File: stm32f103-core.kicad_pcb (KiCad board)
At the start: 2 copper layers, 30 x 35 mm, 31 parts, among them J1 Conn_01x14, J3 Conn_01x12, J4 Conn_01x12, SW1 SW_Push, U1 STM32F103C8T6, U2 AMS1117-3.3, Y1 O8M, Y2 O32.768K

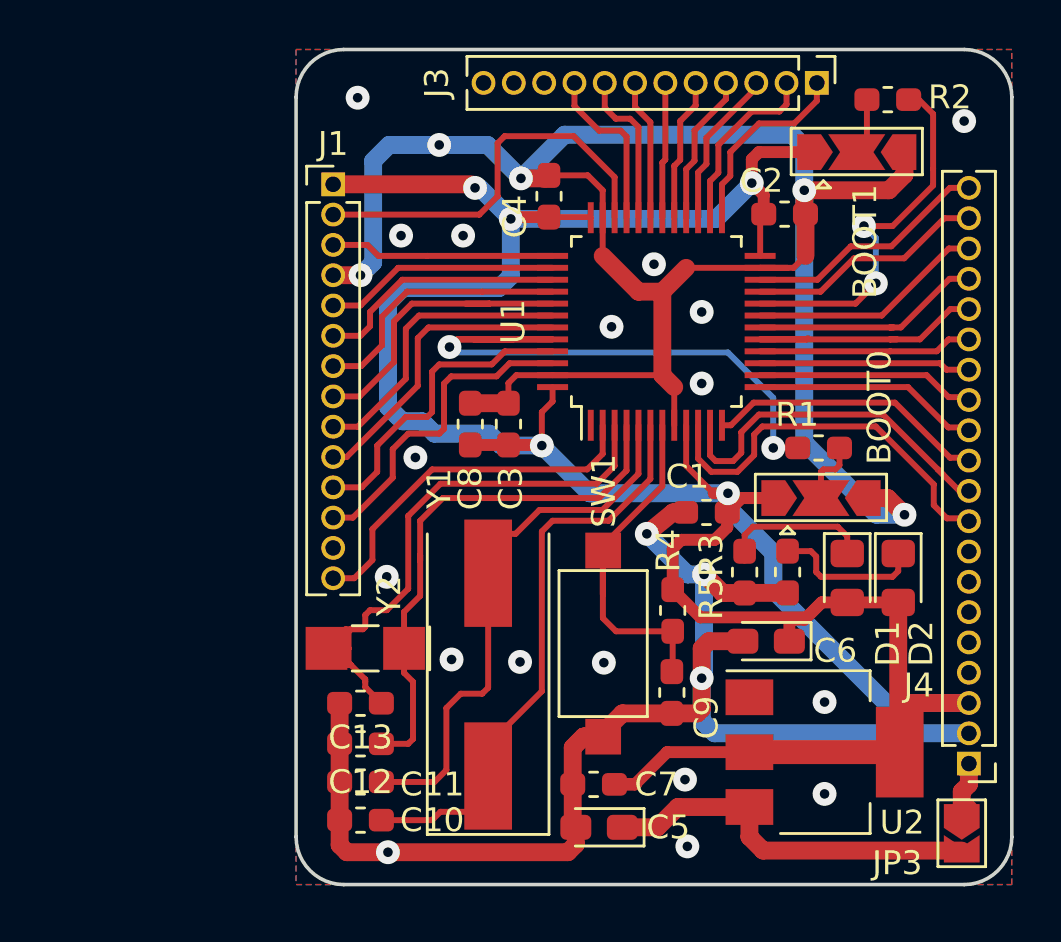
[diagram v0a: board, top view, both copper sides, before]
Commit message: update,
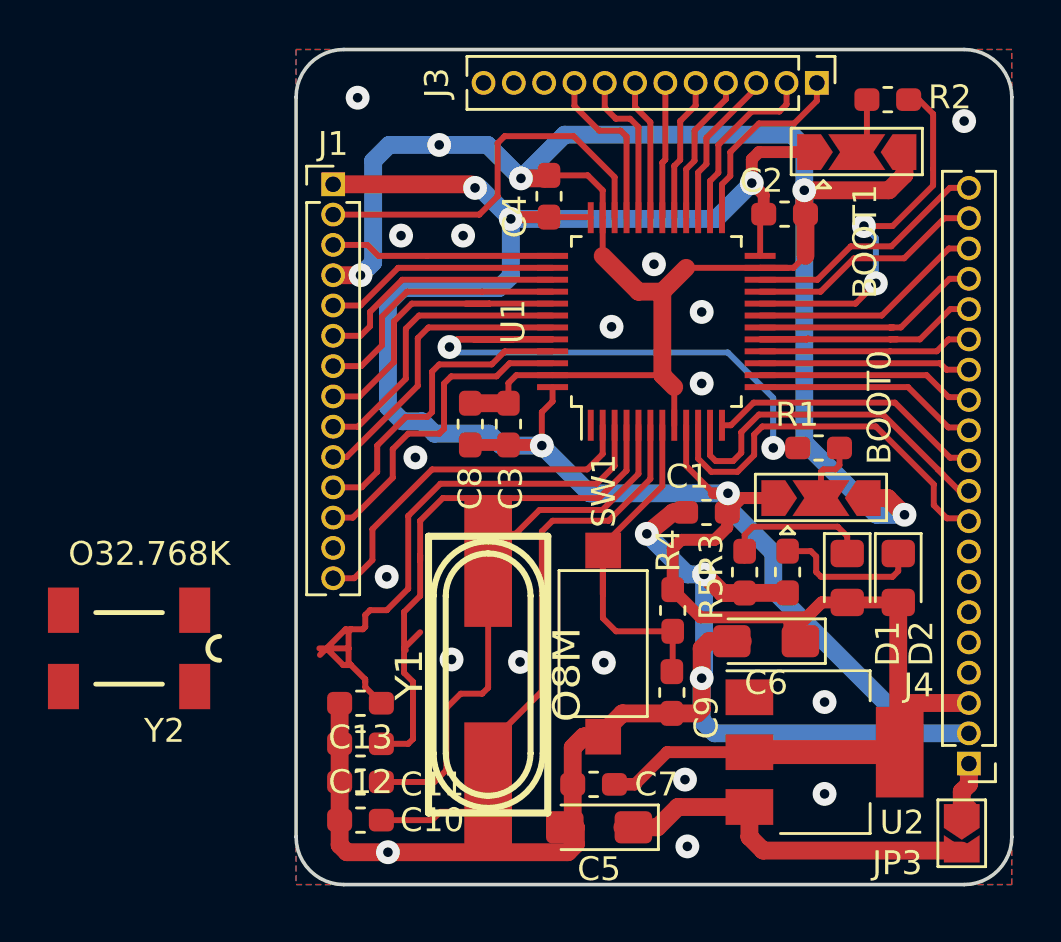
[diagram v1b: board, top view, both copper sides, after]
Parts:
- C5, C6: footprint Capacitor_Tantalum_SMD:CP_EIA-2012-12_Kemet-R_Pad1.30x1.05mm_HandSolder -> Capacitor_Tantalum_SMD:CP_EIA-3216-12_Kemet-S_Pad1.58x1.35mm_HandSolder
- Y1: footprint Crystal:Crystal_SMD_HC49-SD -> w_crystal:hc-49_smd
- Y2: footprint Crystal:Crystal_SMD_MicroCrystal_CC7V-T1A-2Pin_3.2x1.5mm_HandSoldering -> footprint-lib.pretty:MC-306
- moved Y2 9.90 mm to (5.00, 37.1)
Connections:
- net 3V3 renamed +3V3
- J1 pad 13: (no net) -> Net-(J1-Pad13)
- J3 pad 10: (no net) -> Net-(J3-Pad10)
- J3 pad 11: (no net) -> Net-(J3-Pad11)
- J3 pad 12: (no net) -> Net-(J3-Pad12)
- J4 pad 4: (no net) -> Net-(J4-Pad4)
- J4 pad 5: (no net) -> Net-(J4-Pad5)
- J4 pad 6: (no net) -> Net-(J4-Pad6)
- J4 pad 7: (no net) -> Net-(J4-Pad7)
- J4 pad 8: (no net) -> Net-(J4-Pad8)
- U1 pad 1: (no net) -> /VBAT
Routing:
- net 3V3: track 0.00 -> 130.7 mm, vias 0 -> 5
- net +3V3: track 130.7 -> 0.00 mm, vias 5 -> 0
